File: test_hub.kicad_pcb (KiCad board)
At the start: 2 copper layers, 101 parts, among them P1 USB_OTG, P2 5V_SEL, P3 5V_EXT, P4 USB1, P5 USB2, P6 USB3, SW1 RST, SW2 BOOT, U1 USB2514B, U2 MIC550X, U3 stm32f072x, U4 AP2171, U5 AP2171, U6 AP2171, U7 LT6106, U8 LT6106, U9 LT6106, Y1 24MHz

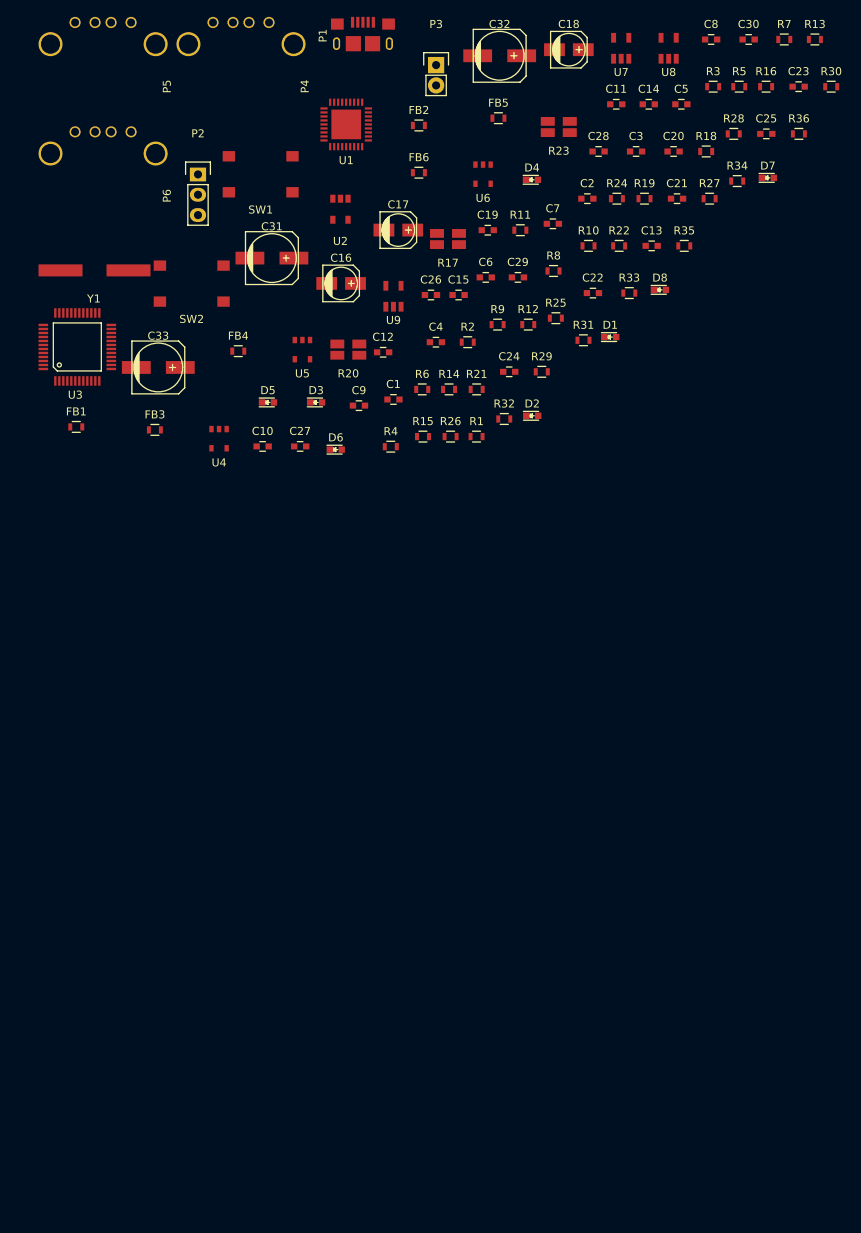
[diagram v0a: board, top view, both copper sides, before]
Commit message: PCB routing done (I think)
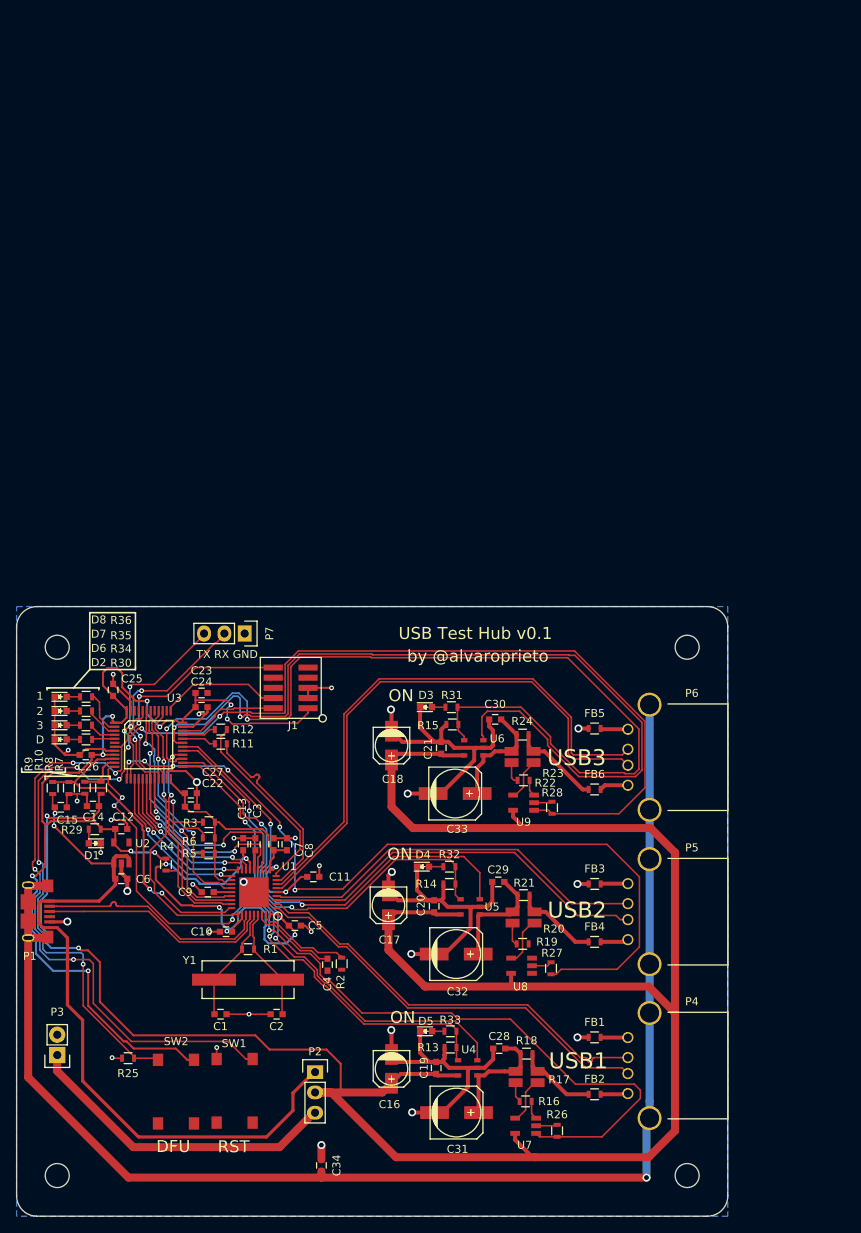
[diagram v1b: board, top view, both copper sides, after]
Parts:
- added C34: 0.1uF, Capacitors_SMD:C_0603, F.Cu at (114.3, 171.4)
- added J1: ARM-SWD, footprints:ARM_SWD_SMD, F.Cu at (110.5, 111.8)
- added P7: UART, Pin_Headers:Pin_Header_Straight_1x03, F.Cu at (104.7, 105.0)
- added REF**: MountingHole_3mm, Mounting_Holes:MountingHole_3mm, F.Cu at (81.3, 106.7)
- added REF**: MountingHole_3mm, Mounting_Holes:MountingHole_3mm, F.Cu at (81.3, 172.7)
- added REF**: MountingHole_3mm, Mounting_Holes:MountingHole_3mm, F.Cu at (160.0, 172.7)
- added REF**: MountingHole_3mm, Mounting_Holes:MountingHole_3mm, F.Cu at (160.0, 106.7)
- moved P4 139.1 mm to (152.6, 159.0), turned to 90 degrees
- moved U7 135.2 mm to (139.8, 166.5), turned to 90 degrees
- moved R13 134.0 mm to (130.4, 156.7), turned to 180 degrees
- moved P3 132.5 mm to (81.3, 157.7), turned to 180 degrees
- moved R16 130.4 mm to (139.8, 163.4), turned to 180 degrees
- moved P5 129.1 mm to (152.6, 139.7), turned to 90 degrees
- moved R7 126.7 mm to (86.8, 124.3), turned to 90 degrees
- moved R30 123.8 mm to (84.9, 118.2)
- moved FB2 123.1 mm to (148.5, 162.6)
- moved R5 116.5 mm to (100.2, 132.4), turned to 180 degrees
- moved P1 116.3 mm to (77.6, 139.7), turned to 270 degrees
- moved U8 116.1 mm to (139.3, 146.5), turned to 90 degrees
- moved R18 115.0 mm to (139.9, 157.5)
- moved SW1 114.6 mm to (103.5, 162.1), turned to 90 degrees
- moved C8 113.7 mm to (110.0, 131.3), turned to 270 degrees
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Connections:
- net /DM4 renamed /USB4_N
- net /DM_IN renamed /USB_UP_N
- net /DN1 renamed /USB1_N
- net /DN2 renamed /USB2_N
- net /DN3 renamed /USB3_N
- net /DP1 renamed /USB1_P
- net /DP2 renamed /USB2_P
- net /DP3 renamed /USB3_P
- net /DP4 renamed /USB4_P
- net /DP_IN renamed /USB_UP_P
- P1 pad 6: GND -> GNDPWR
- P4 pad 5: Net-(FB1-Pad2) -> GNDPWR
- P5 pad 5: Net-(FB3-Pad2) -> GNDPWR
- P6 pad 5: Net-(FB5-Pad2) -> GNDPWR
- R25 pad 2: +3V3 -> GND
- U1 pad 20: /PRTPWR4 -> Net-(U1-Pad20)
- U1 pad 21: /OCS_N4 -> +3V3
- U3 pad 15: Net-(U3-Pad15) -> /OCS_N3
- U3 pad 16: Net-(U3-Pad16) -> /PRTPWR3
- U3 pad 17: Net-(U3-Pad17) -> /OCS_N2
- U3 pad 18: /PRTPWR1 -> /PRTPWR2
- U3 pad 19: /PRTPWR2 -> /OCS_N1
- U3 pad 2: /5V_FLG1 -> /LED0
- U3 pad 20: /PRTPWR3 -> /PRTPWR1
- U3 pad 21: /PRTPWR4 -> /USART3_TX
- U3 pad 22: /OCS_N1 -> /USART3_RX
- U3 pad 25: /OCS_N2 -> /5V_EN1
- U3 pad 26: /OCS_N3 -> /5V_EN2
- U3 pad 27: /OCS_N4 -> /5V_EN3
- U3 pad 28: /DBG_LED -> /HUB_RST_N
- U3 pad 29: /LED0 -> /5V_FLG1
- U3 pad 3: /5V_FLG2 -> /LED1
- U3 pad 30: /LED1 -> /5V_FLG2
- U3 pad 31: /LED2 -> /5V_FLG3
- U3 pad 34: /5V_EN1 -> /SWDIO
- U3 pad 37: /5V_EN2 -> /SWCLK
- U3 pad 38: /5V_EN3 -> Net-(U3-Pad38)
- U3 pad 4: /5V_FLG3 -> /LED2
- U3 pad 41: /HUB_RST_N -> Net-(U3-Pad41)
- U3 pad 5: Net-(U3-Pad5) -> /DBG_LED
- U7 pad 5: +5V -> /5V_OUT
- U8 pad 5: +5V -> /5V_OUT
- U9 pad 5: +5V -> /5V_OUT
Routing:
- net /5V_OUT: track 0.00 -> 293.7 mm, vias 0 -> 2
- net +3V3: track 0.00 -> 235.0 mm, vias 0 -> 17
- net GND: track 0.00 -> 202.7 mm, vias 0 -> 30
- net GNDPWR: track 0.00 -> 171.7 mm, vias 0 -> 1
- net /5V_EN3: track 0.00 -> 116.5 mm, vias 0 -> 2
- net /SNS1: track 0.00 -> 112.4 mm, vias 0 -> 4
- net /5V_FLG3: track 0.00 -> 109.3 mm, vias 0 -> 2
- net /SNS3: track 0.00 -> 105.8 mm, vias 0 -> 2
- net /SNS2: track 0.00 -> 101.9 mm, vias 0 -> 6
- net /nRST: track 0.00 -> 99.2 mm, vias 0 -> 6
- net +5V: track 0.00 -> 92.6 mm, vias 0 -> 2
- net /USB3_N: track 0.00 -> 69.5 mm
- net /USB3_P: track 0.00 -> 69.3 mm
- net /BOOT0: track 0.00 -> 67.9 mm, vias 0 -> 6
- net /5V_FLG1: track 0.00 -> 63.5 mm, vias 0 -> 2
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- added copper zone on B.Cu, net GND
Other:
- board outline added: 88.9 x 76.2 mm
- net class Default: clearance 0.2 -> 0.16; trace_width 0.25 -> 0.13; via_drill 0.4 -> 0.305
- rule trace_clearance: 0.2 -> 0.16
- rule trace_min: 0.2 -> 0.13
- rule via_min_drill: 0.3 -> 0.305
- rule via_min_size: 0.4 -> 0.6
- board text added: "1"
- board text added: "2"
- board text added: "3"
- board text added: "D"
- board text added: "DFU"
- board text added: "ON"
- board text added: "RST"
- board text added: "TX RX GND"
- board text added: "USB Test Hub v0.1"
- board text added: "USB1"
- board text added: "USB2"
- board text added: "USB3"
- board text added: "by @alvaroprieto"
